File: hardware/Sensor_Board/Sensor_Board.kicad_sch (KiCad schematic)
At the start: 0 parts

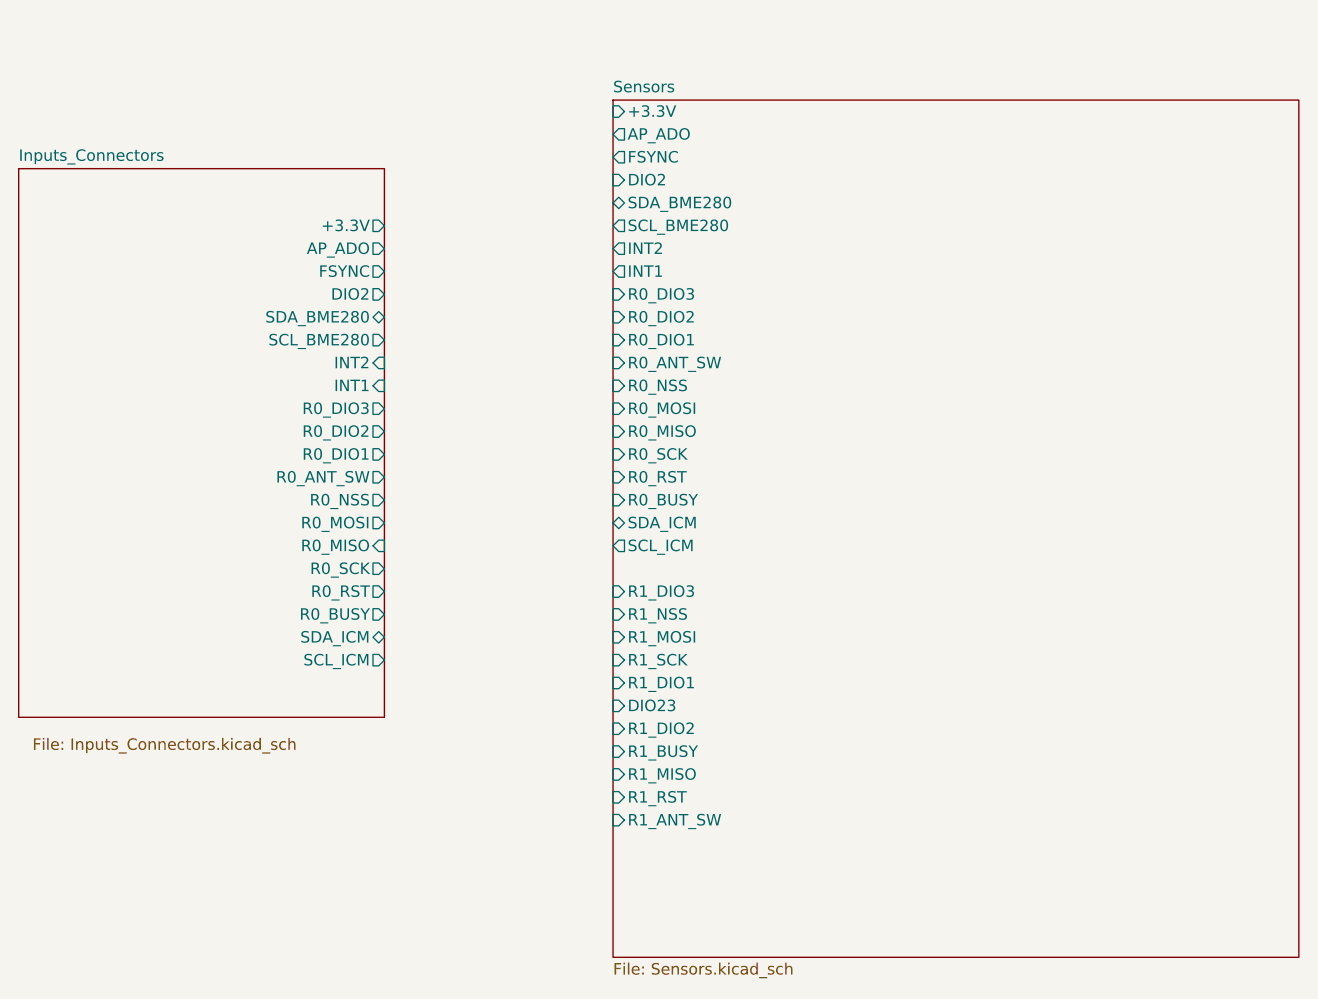
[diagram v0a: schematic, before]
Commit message: feat(Hw):floorplans_updated
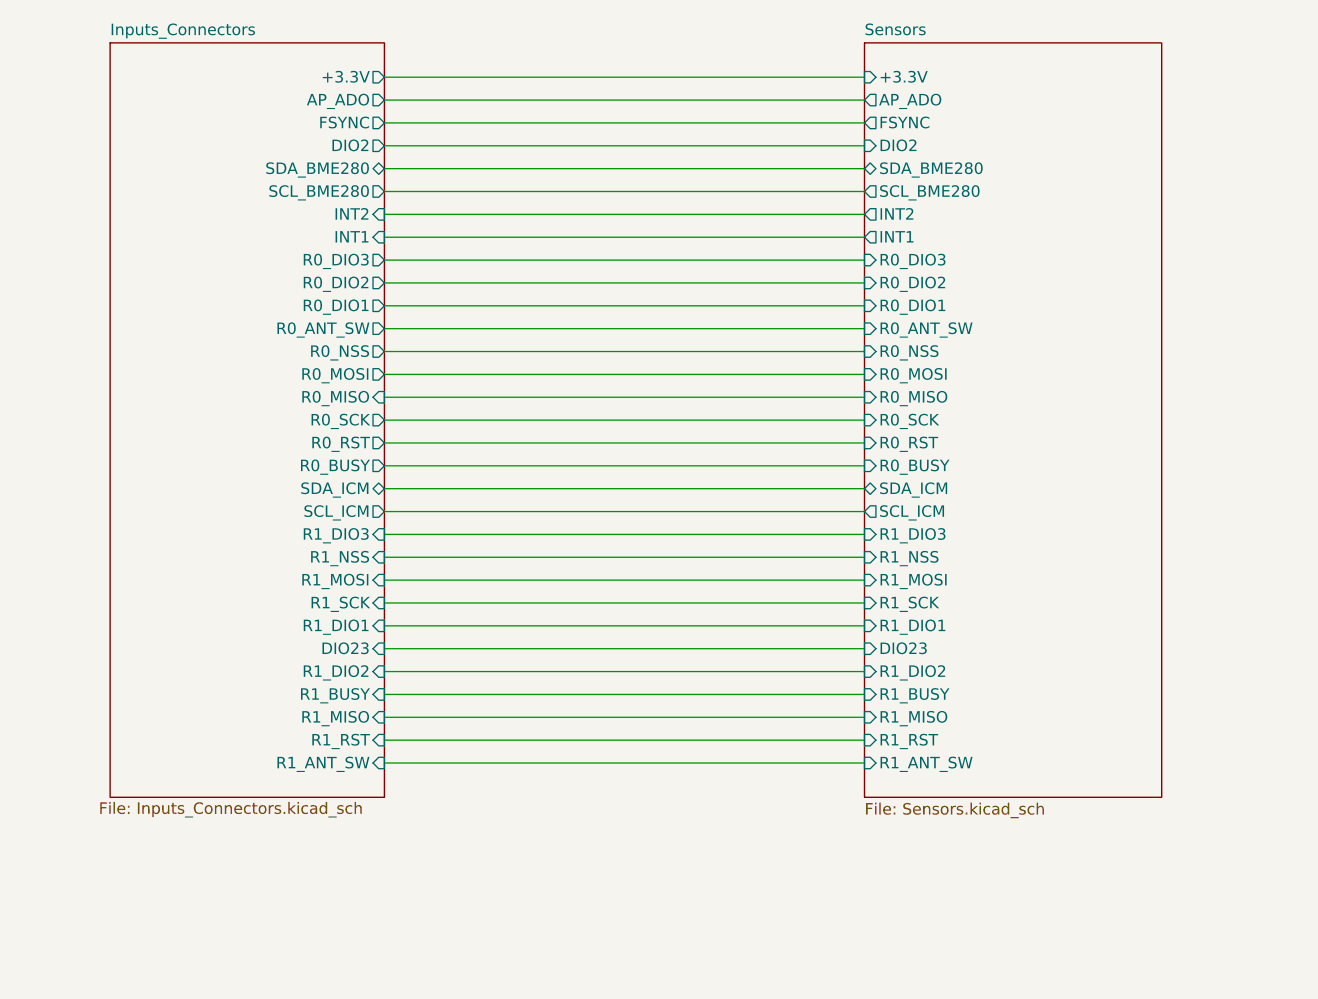
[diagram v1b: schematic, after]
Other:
- sheet Inputs_Connectors ports: added DIO23, R1_ANT_SW, R1_BUSY, R1_DIO1, R1_DIO2, R1_DIO3, R1_MISO, R1_MOSI, R1_NSS, R1_RST, R1_SCK; removed none
